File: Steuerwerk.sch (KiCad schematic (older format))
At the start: 112 parts

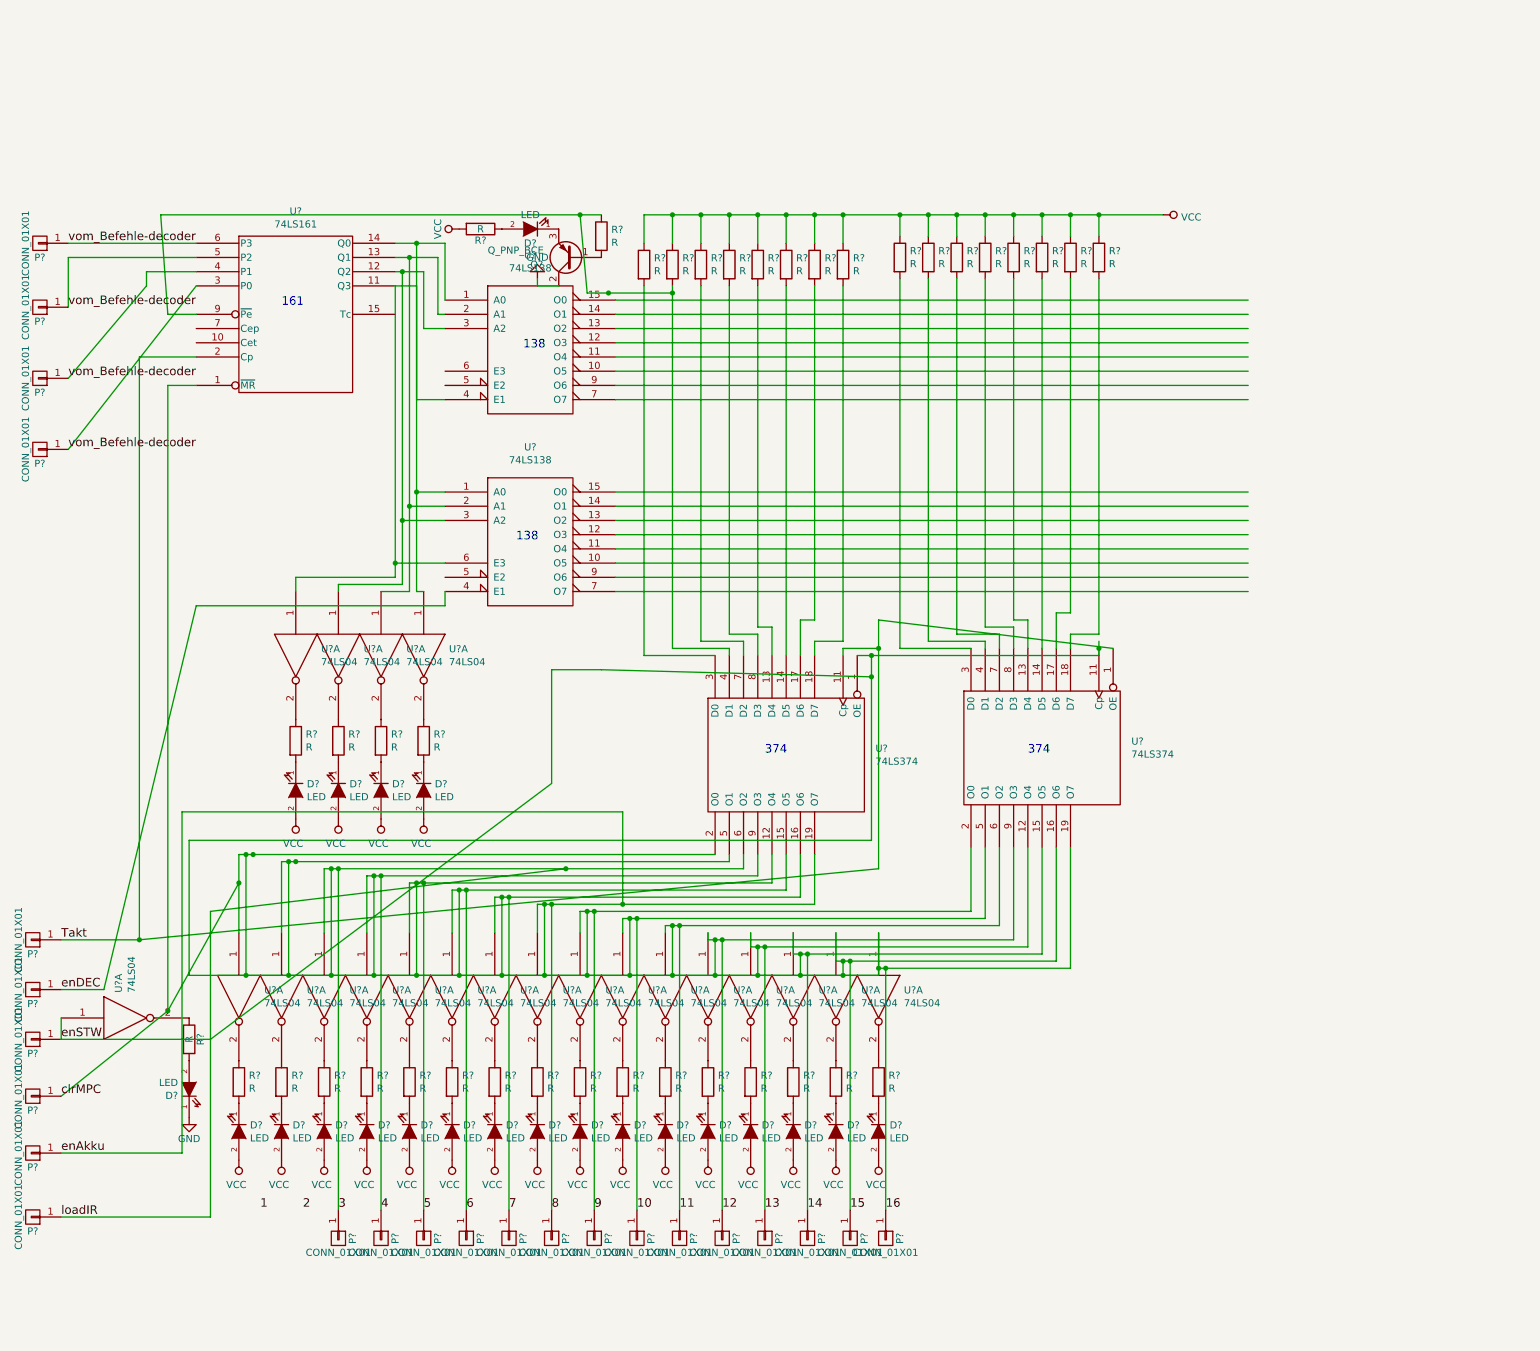
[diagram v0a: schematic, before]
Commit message: Annotierung und Footprints
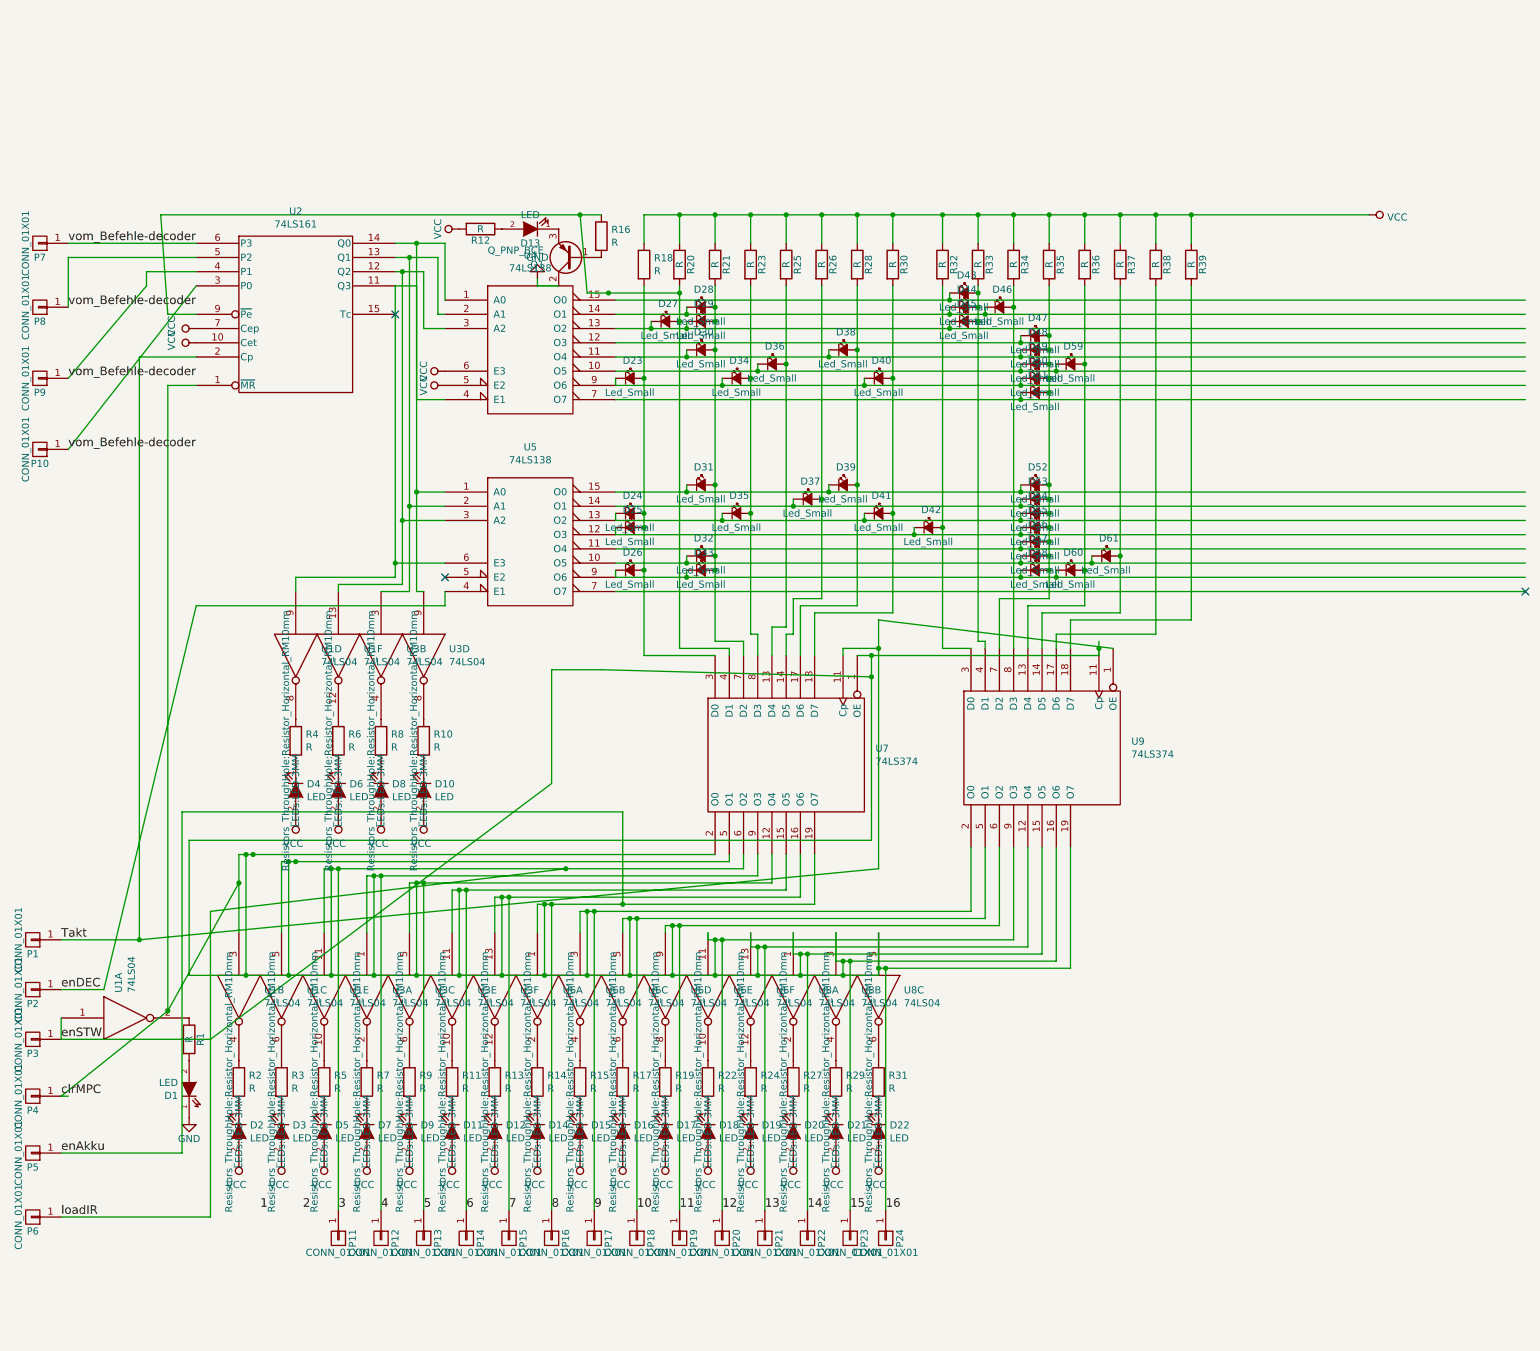
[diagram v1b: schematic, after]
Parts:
- removed R? (x15): R, symbol R
- added D23, D24, D25, D26, D27, D28, D29, D30, D31, D32, D33, D34, D35, D36, D37, D38, D39, D40, D41, D42, D43, D44, D45, D46, D47, D48, D49, D50, D51, D52, D53, D54, D55, D56, D57, D58, D59, D60, D61: Led_Small, symbol Led_Small
- added R20, R21, R23, R25, R26, R28, R30, R32, R33, R34, R35, R36, R37, R38, R39: R, symbol R
- D10, D11, D12, D14, D15, D16, D17, D18, D19, D2, D20, D21, D22, D3, D4, D5, D6, D7, D8, D9: renamed from D?; footprint (none) -> LEDs:LED-3MM
- R10, R11, R13, R14, R15, R17, R19, R2, R22, R24, R27, R29, R3, R31, R4, R5, R6, R7, R8, R9: renamed from R?; footprint (none) -> Resistors_ThroughHole:Resistor_Horizontal_RM10mm
- gave numbers to parts that had none: 40
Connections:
- wire segments 303 -> 269
- no-connect marks 0 -> 3
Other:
- note removed: "138"
- note removed: "161"
- note removed: "374"

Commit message: Steuerwerk: Footprints
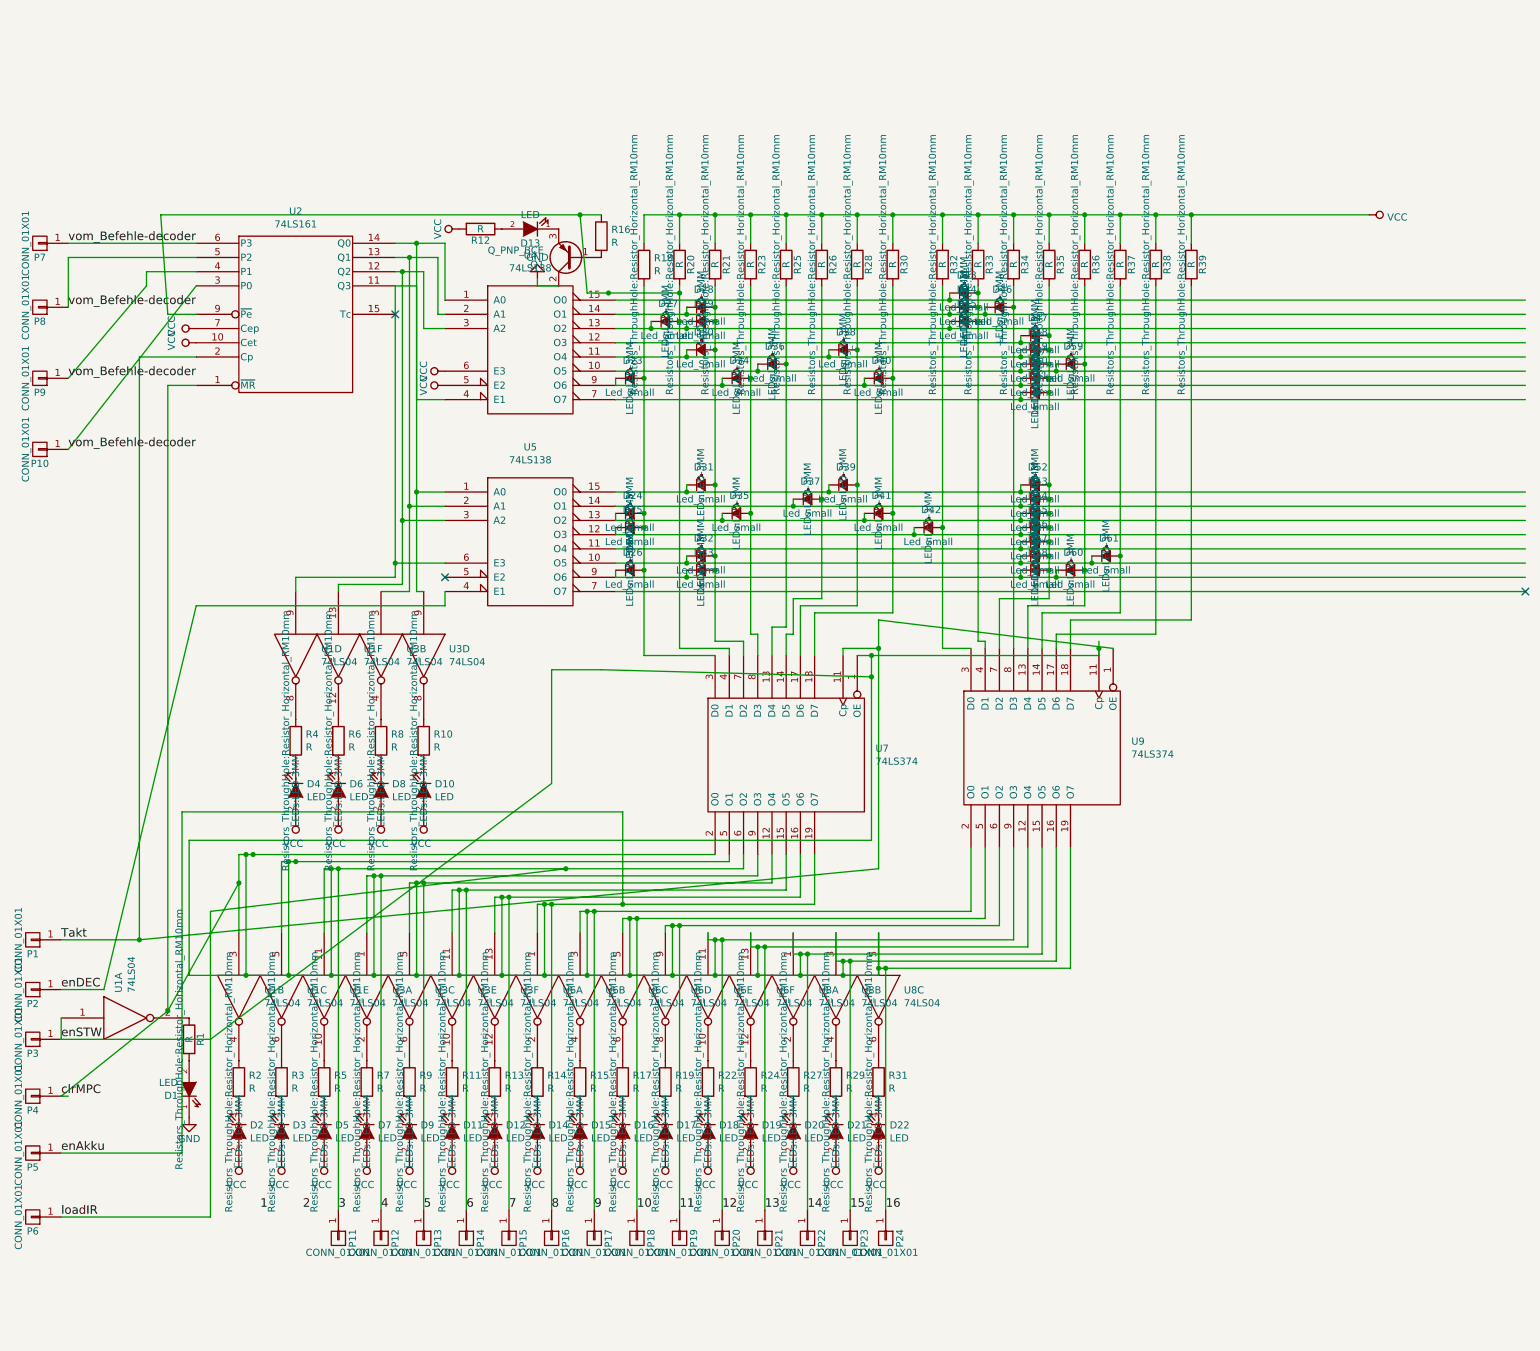
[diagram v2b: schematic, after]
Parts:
- D13, D23, D24, D25, D26, D27, D28, D31, D32, D33, D34, D35, D36, D37, D38, D39, D40, D41, D42, D43, D44, D45, D46, D47, D48, D49, D50, D51, D52, D53, D54, D55, D56, D57, D58, D59, D60, D61: footprint (none) -> LEDs:LED-3MM
- R1, R12, R18, R20, R21, R23, R25, R26, R28, R30, R32, R33, R34, R35, R36, R37, R38, R39: footprint (none) -> Resistors_ThroughHole:Resistor_Horizontal_RM10mm

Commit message: Footprints Steuerwerk
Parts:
- P10: footprint (none) -> Connect:1pin
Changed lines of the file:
@@
 F 0 "P10" H 700 2250 50  0000 C CNN
 F 1 "CONN_01X01" V 800 2150 50  0000 C CNN
-F 2 "" H 700 2150 50  0001 C CNN
+F 2 "Connect:1pin" H 700 2150 50  0001 C CNN
 F 3 "" H 700 2150 50  0000 C CNN
 	1    700  2150
